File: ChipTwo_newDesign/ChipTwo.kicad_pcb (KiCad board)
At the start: 4 copper layers, 113 x 113.8 mm, 27 parts

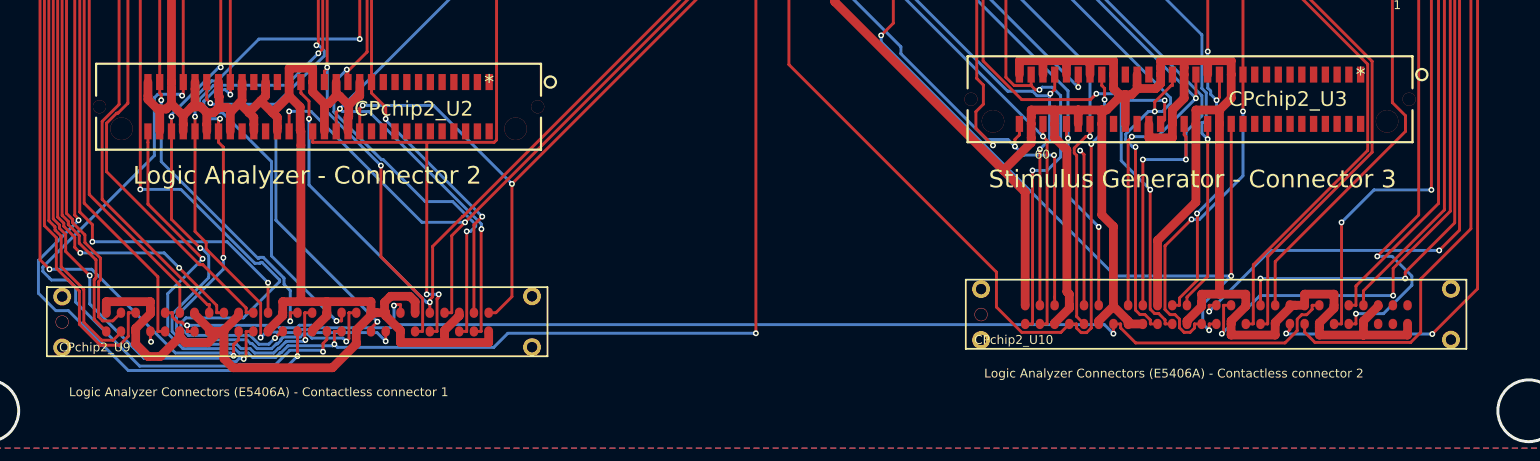
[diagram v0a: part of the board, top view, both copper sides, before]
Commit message: Changes finilised
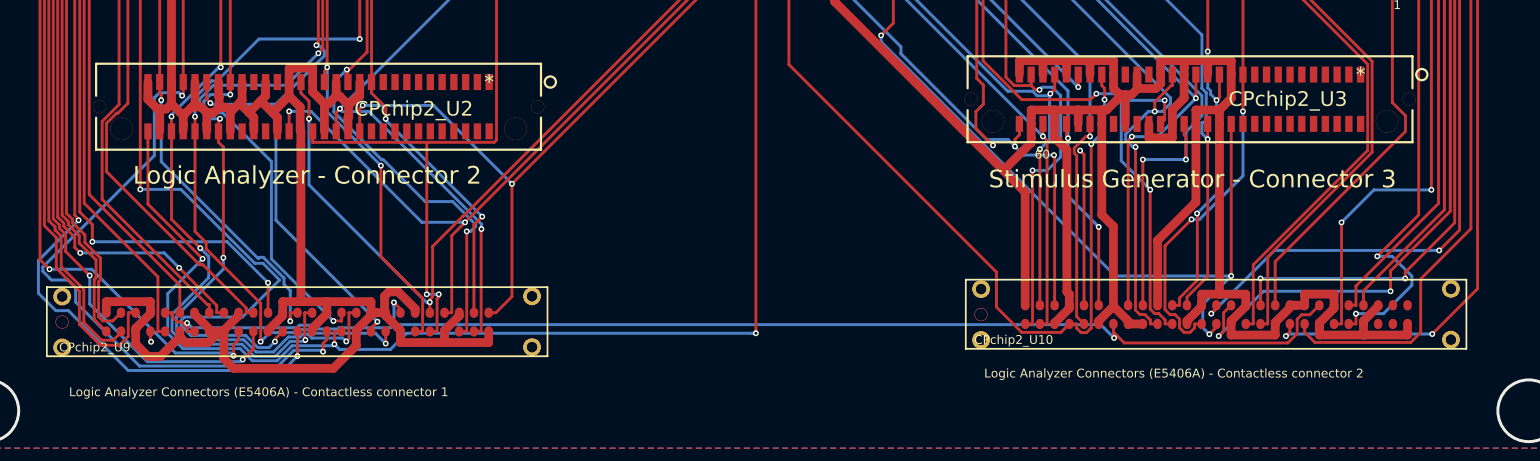
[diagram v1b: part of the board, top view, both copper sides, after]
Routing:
- net clk: track 212.7 -> 214.0 mm
- net io[14]: track 78.5 -> 79.0 mm
